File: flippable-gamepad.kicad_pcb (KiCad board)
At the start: 2 copper layers, 228.6 x 100 mm, 87 parts

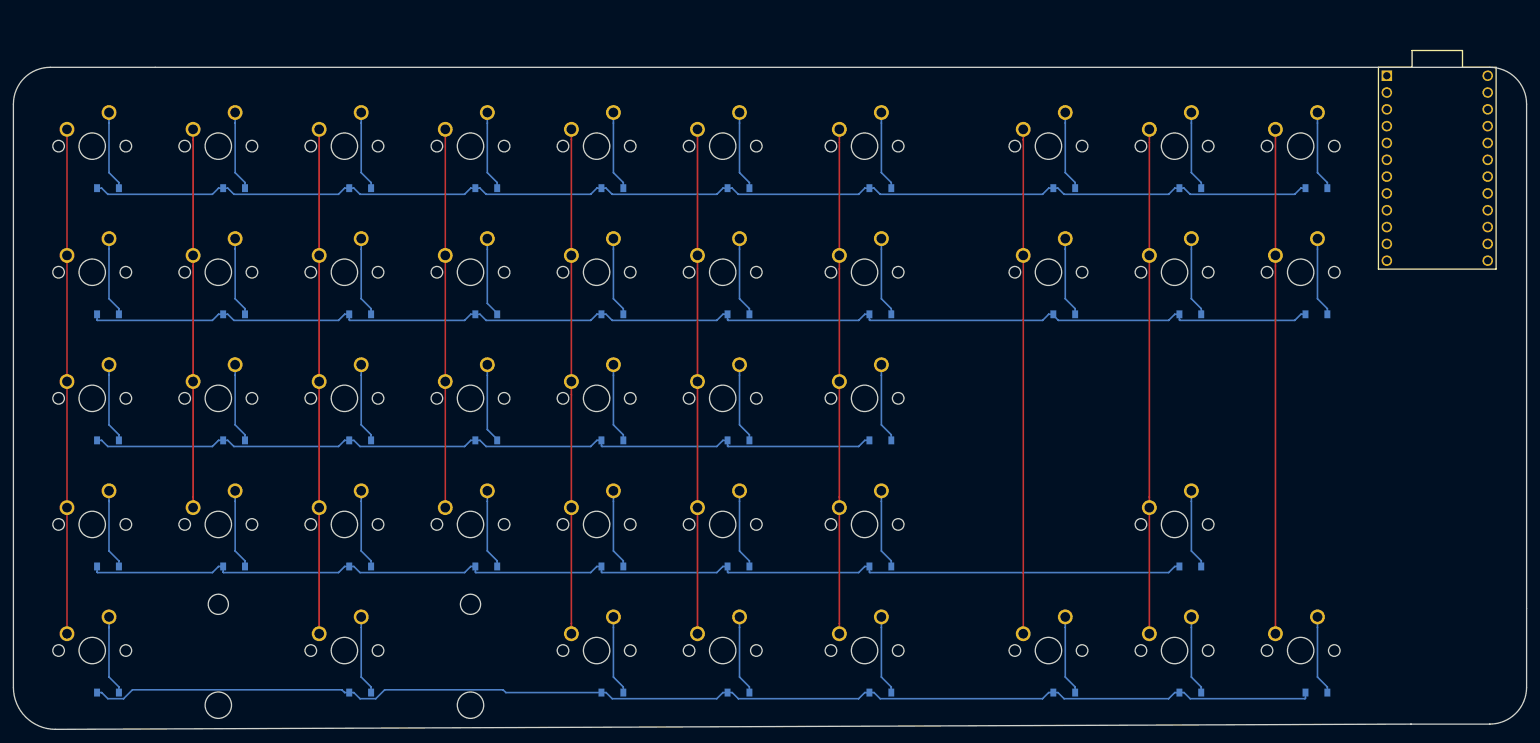
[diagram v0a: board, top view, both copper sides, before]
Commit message: Fresh start
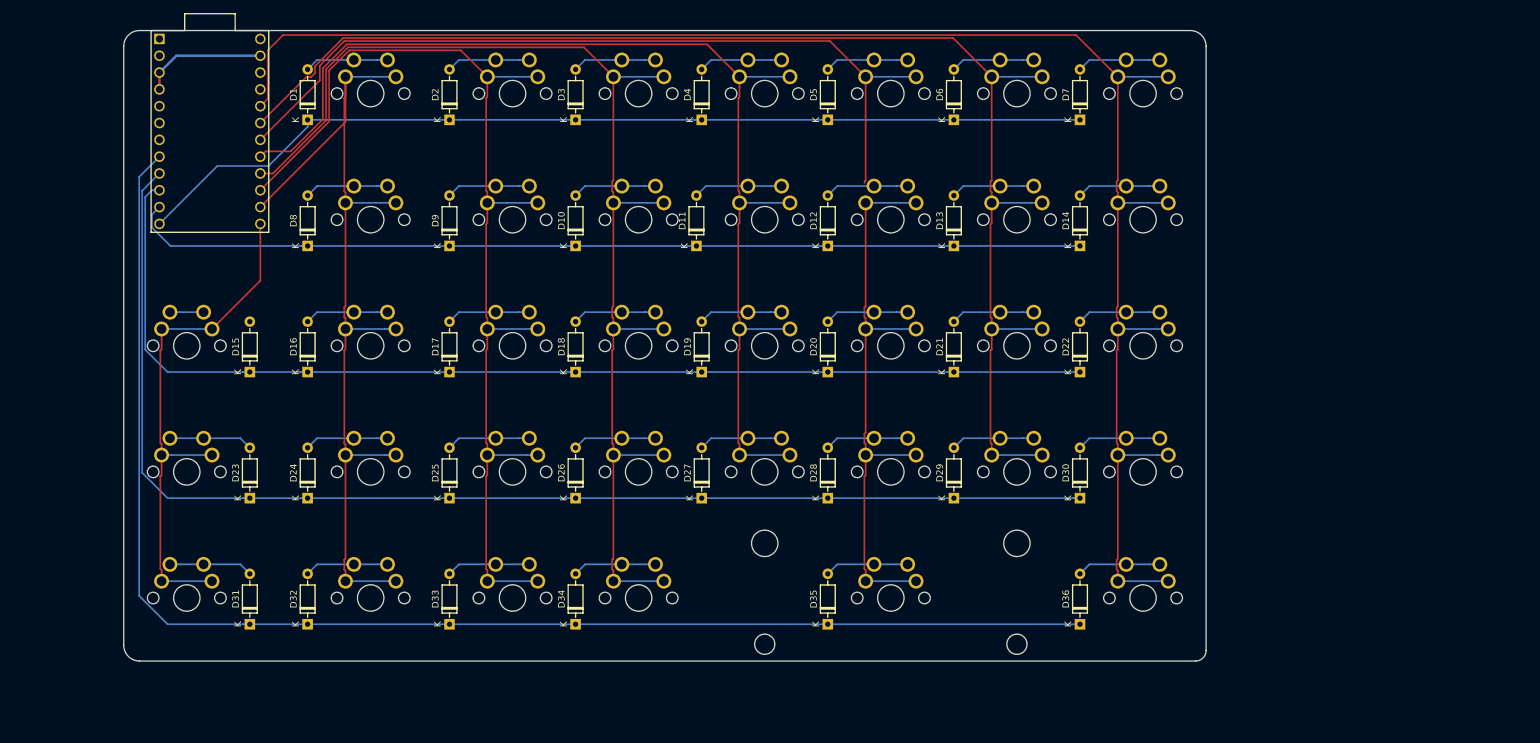
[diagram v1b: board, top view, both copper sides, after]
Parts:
- removed D37, D38, D39, D40, D41, D42, D43: D_Small, Diode_SMD:D_SOD-123
- removed MX37: MX-NoLED, MX_Only:MXOnly-3U-NoLED
- removed MX38, MX39, MX41, MX42, MX43: MX-NoLED, MX_Only:MXOnly-1U-NoLED
- removed MX40: MX-NoLED, MX_Only:MXOnly-1.25U-NoLED
- D1, D10, D11, D12, D13, D14, D15, D16, D17, D18, D19, D2, D20, D21, D22, D23, D24, D25, D26, D27, D28, D29, D3, D30, D31, D32, D33, D34, D35, D36, D4, D5, D6, D7, D8, D9: footprint Diode_SMD:D_SOD-123 -> Diode_THT:D_DO-35_SOD27_P7.62mm_Horizontal; moved to F.Cu
- MX1, MX16, MX24, MX32, MX8: footprint MX_Only:MXOnly-1U-NoLED -> MX_Only:MXOnly-1.25U-Reversible-NoLED
- MX10, MX11, MX12, MX13, MX14, MX15, MX18, MX19, MX2, MX20, MX21, MX22, MX23, MX25, MX26, MX28, MX29, MX3, MX30, MX31, MX33, MX36, MX4, MX5, MX6, MX9: footprint MX_Only:MXOnly-1U-NoLED -> MX_Only:MXOnly-1U-Reversible-NoLED
- MX17, MX27, MX34, MX7: footprint MX_Only:MXOnly-1.25U-NoLED -> MX_Only:MXOnly-1U-Reversible-NoLED
- MX35: footprint MX_Only:MXOnly-1U-NoLED -> MX_Only:MXOnly-3U-Reversible-ReversedStabilizers-NoLED
- moved ProMicro1 185.5 mm to (67.0, 54.9)
- moved MX36 158.9 mm to (208.0, 125.4)
- moved D36 147.2 mm to (198.4, 129.4), turned to 90 degrees
- moved MX21 139.9 mm to (188.9, 87.3)
- moved MX22 139.9 mm to (208.0, 87.3)
- moved D22 128.2 mm to (198.4, 91.3), turned to 90 degrees
- moved D21 128.2 mm to (179.4, 91.3), turned to 90 degrees
- moved MX29 120.9 mm to (188.9, 106.4)
- moved MX28 120.9 mm to (169.9, 106.4)
- moved MX30 120.9 mm to (208.0, 106.4)
- moved D8 114.6 mm to (81.8, 72.2), turned to 90 degrees
- moved D10 112.3 mm to (122.2, 72.2), turned to 90 degrees
- moved D9 112.3 mm to (103.2, 72.2), turned to 90 degrees
- moved D28 109.2 mm to (160.3, 110.3), turned to 90 degrees
- moved D30 109.2 mm to (198.4, 110.3), turned to 90 degrees
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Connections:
- D10 pad 1: ROW0 -> ROW1
- D15 pad 1: ROW1 -> ROW2
- D16 pad 1: ROW1 -> ROW2
- D17 pad 1: ROW1 -> ROW2
- D18 pad 1: ROW1 -> ROW2
- D19 pad 1: ROW1 -> ROW2
- D20 pad 1: ROW1 -> ROW2
- D23 pad 1: ROW2 -> ROW3
- D24 pad 1: ROW2 -> ROW3
- D25 pad 1: ROW2 -> ROW3
- D26 pad 1: ROW2 -> ROW3
- D27 pad 1: ROW2 -> ROW3
- D31 pad 1: ROW3 -> ROW4
- D32 pad 1: ROW3 -> ROW4
- D33 pad 1: ROW3 -> ROW4
- D34 pad 1: ROW3 -> ROW4
- D35 pad 1: ROW3 -> ROW4
- D8 pad 1: ROW0 -> ROW1
- D9 pad 1: ROW0 -> ROW1
- MX1 pad 1: COL0 -> COL1
- MX10 pad 1: COL9 -> COL3
- MX11 pad 1: COL0 -> COL4
- MX12 pad 1: COL1 -> COL5
- MX13 pad 1: COL2 -> COL6
- MX14 pad 1: COL3 -> COL7
- MX15 pad 1: COL4 -> COL0
- MX16 pad 1: COL5 -> COL1
- MX17 pad 1: COL6 -> COL2
- MX18 pad 1: COL7 -> COL3
- MX19 pad 1: COL8 -> COL4
- MX2 pad 1: COL1 -> COL2
- MX20 pad 1: COL9 -> COL5
- MX21 pad 1: COL0 -> COL6
- MX22 pad 1: COL1 -> COL7
- MX23 pad 1: COL2 -> COL0
- MX24 pad 1: COL3 -> COL1
- MX25 pad 1: COL4 -> COL2
- MX26 pad 1: COL5 -> COL3
- MX27 pad 1: COL6 -> COL4
- MX28 pad 1: COL0 -> COL5
- MX29 pad 1: COL1 -> COL6
- MX3 pad 1: COL2 -> COL3
- MX30 pad 1: COL2 -> COL7
- MX31 pad 1: COL3 -> COL0
- MX32 pad 1: COL4 -> COL1
- MX33 pad 1: COL5 -> COL2
- MX34 pad 1: COL6 -> COL3
- MX35 pad 1: COL8 -> COL5
- MX36 pad 1: COL0 -> COL7
- MX4 pad 1: COL3 -> COL4
- MX5 pad 1: COL4 -> COL5
- MX6 pad 1: COL5 -> COL6
- MX7 pad 1: COL6 -> COL7
- MX8 pad 1: COL7 -> COL1
- MX9 pad 1: COL8 -> COL2
- ProMicro1 pad 10: Net-(ProMicro1-Pad10) -> ROW2
- ProMicro1 pad 11: Net-(ProMicro1-Pad11) -> ROW1
- ProMicro1 pad 12: Net-(ProMicro1-Pad12) -> ROW0
- ProMicro1 pad 13: Net-(ProMicro1-Pad13) -> COL0
- ProMicro1 pad 14: Net-(ProMicro1-Pad14) -> COL1
- ProMicro1 pad 15: Net-(ProMicro1-Pad15) -> COL2
- ProMicro1 pad 16: Net-(ProMicro1-Pad16) -> COL3
- ProMicro1 pad 17: Net-(ProMicro1-Pad17) -> COL4
- ProMicro1 pad 18: Net-(ProMicro1-Pad18) -> COL5
- ProMicro1 pad 19: Net-(ProMicro1-Pad19) -> COL6
- ProMicro1 pad 20: Net-(ProMicro1-Pad20) -> COL7
- ProMicro1 pad 8: Net-(ProMicro1-Pad8) -> ROW4
- ProMicro1 pad 9: Net-(ProMicro1-Pad9) -> ROW3
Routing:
- net COL7: track 76.2 -> 255.8 mm
- net COL5: track 76.2 -> 213.0 mm
- net COL6: track 76.2 -> 206.9 mm
- net COL3: track 57.2 -> 182.5 mm
- net COL4: track 76.2 -> 174.0 mm
- net COL2: track 76.2 -> 164.1 mm
- net COL1: track 57.2 -> 139.9 mm
- net COL9: track 76.2 -> 0.00 mm
- net COL8: track 76.2 -> 0.00 mm
- net ROW1: track 192.0 -> 144.9 mm
- net ROW2: track 122.3 -> 168.3 mm
- net ROW0: track 189.5 -> 146.2 mm
- net ROW4: track 189.1 -> 211.5 mm
- net GND: track 0.00 -> 18.8 mm
- net ROW3: track 171.9 -> 189.6 mm
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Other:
- board size 228.6 x 100 mm -> 163.5 x 95.3 mm
- net class Default: trace_width 0.25 -> 0.254
- net class Power added: clearance 0.2, trace_width 0.381, via_dia 0.8, via_drill 0.4
